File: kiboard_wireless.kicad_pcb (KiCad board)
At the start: 2 copper layers, 237.1 x 98.8 mm, 117 parts, among them J1 USB_C_Receptacle_USB2.0_16P, J2 Conn_01x02_Shielded, J3 TC2030_SWD, Q1 2N7002, SW1 SW_Nidec_CAS-120A1, SW2 SW_Push_45deg, U1 nRF52840_E73-2G4M08S1C, U3 BQ24075RGT, U4 MAX17048, U5 SRV05-4

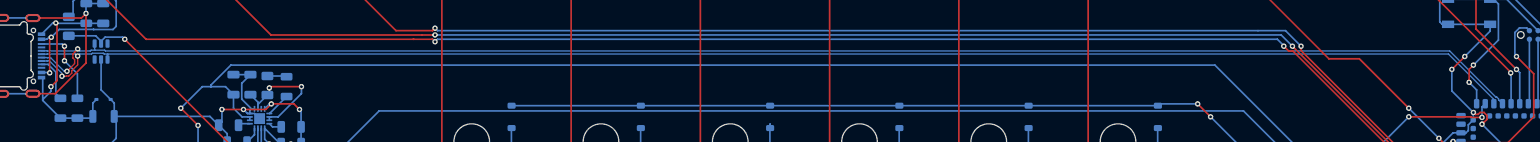
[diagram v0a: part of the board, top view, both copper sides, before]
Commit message: improvements
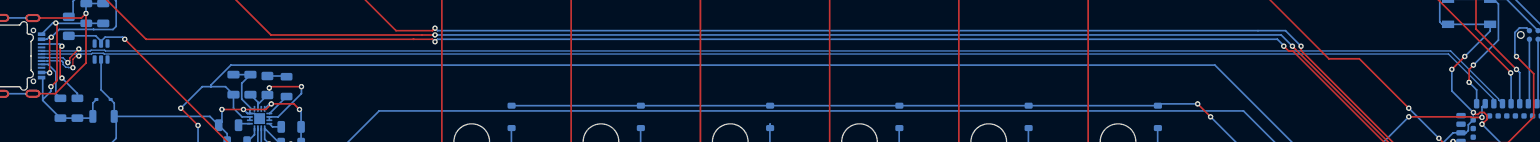
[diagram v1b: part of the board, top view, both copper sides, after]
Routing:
- net usb-D+: track 228.7 -> 225.8 mm
- net usb-D-: track 227.3 -> 225.4 mm
